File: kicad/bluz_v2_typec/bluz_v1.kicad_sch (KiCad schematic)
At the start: 76 parts, among them J10 Conn, J11 Conn, J12 BTAnt, J2 Conn, J3 Conn, J4 Conn, J5 Conn, J6 Conn, J7 Conn, J8 Conn, J9 USB_C_Receptacle_PowerOnly_6P, M1 Z3OC1T8219731, Q2 RUM002N05, SW1 SW_DPDT_x2, U1 MCP73831, U3 TLV3201AIDCK, U4 AP3015KTR, U5 MCP1700-1.8, U6 PAM8904EGPR, U7 TPS627451DSSR, Y1 NX1612SA-32MHz, Y2 NX2012SA-32.768

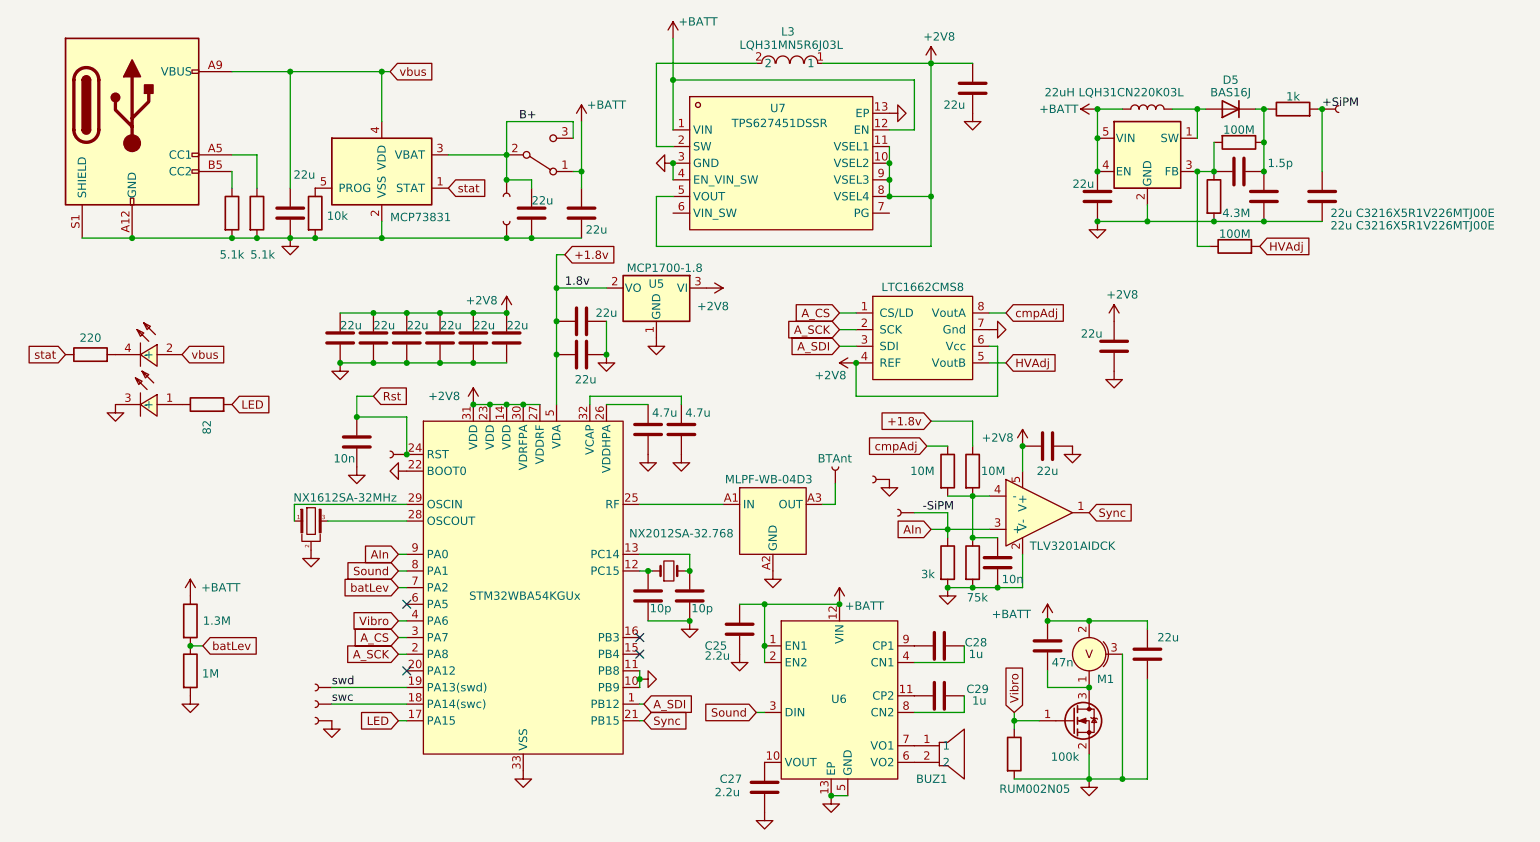
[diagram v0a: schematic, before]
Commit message: изменено:      Android/BluZ_v2/BluZ/Android/BluZ_LPM/BluZ/src/main/java/ru/starline/bluz/SettingsFragment.kt 	новый файл:    kicad/bluz_v1_LED/2024-05-07_07-39-39.kicad_sym 	новый файл:    kicad/bluz_v1_LED/CSPG6_1P05X1P65_STM-L.kicad_mod 	новый файл:    kicad/bluz_v1_LED/CSPG6_1P05X1P65_STM-M.kicad_mod 	новый файл:    kicad/bluz_v1_LED/CSPG6_1P05X1P65_STM.kicad_mod 	новый файл:    kicad/bluz_v1_LED/bluz_v1-backups/bluz_v1-2026-07-10_154057.zip 	новый файл:    kicad/bluz_v1_LED/bluz_v1-backups/bluz_v1-2026-07-10_154720.zip 	новый файл:    kicad/bluz_v1_LED/bluz_v1-backups/bluz_v1-2026-07-13_101334.zip 	новый файл:    kicad/bluz_v1_LED/bluz_v1-backups/bluz_v1-2026-07-13_113755.zip 	новый файл:    kicad/bluz_v1_LED/bluz_v1-backups/bluz_v1-2026-09-14_165340.zip 	новый файл:    kicad/bluz_v1_LED/bluz_v1-backups/bluz_v1-2026-09-14_165908.zip 	новый файл:    kicad/bluz_v1_LED/bluz_v1-backups/bluz_v1-2026-09-14_170418.zip 	новый файл:    kicad/bluz_v1_LED/bluz_v1-backups/bluz_v1-2026-09-14_174516.zip 	новый файл:    kicad/bluz_v1_LED/bluz_v1-backups/bluz_v1-2026-09-14_181225.zip 	новый файл:    kicad/bluz_v1_LED/bluz_v1-backups/bluz_v1-2026-09-15_141616.zip 	новый файл:    kicad/bluz_v1_LED/bluz_v1-backups/bluz_v1-2026-09-15_144107.zip 	новый файл:    kicad/bluz_v1_LED/bluz_v1-backups/bluz_v1-2026-09-15_145150.zip 	новый файл:    kicad/bluz_v1_LED/bluz_v1-backups/bluz_v1-2026-09-15_150420.zip 	новый файл:    kicad/bluz_v1_LED/bluz_v1-backups/bluz_v1-2026-09-15_155235.zip 	новый файл:    kicad/bluz_v1_LED/bluz_v1-backups/bluz_v1-2026-09-17_183048.zip 	новый файл:    kicad/bluz_v1_LED/bluz_v1-backups/bluz_v1-2026-09-17_183700.zip 	новый файл:    kicad/bluz_v1_LED/bluz_v1-backups/bluz_v1-2026-09-17_184420.zip 	новый файл:    kicad/bluz_v1_LED/bluz_v1-backups/bluz_v1-2026-09-17_185211.zip 	новый файл:    kicad/bluz_v1_LED/bluz_v1-backups/bluz_v1-2026-09-17_190709.zip 	новый файл:    kicad/bluz_v1_LED/bluz_v1-backups/bluz_v1-2026-09-18_172926.zip 	новый файл:    kicad/bluz_v1_L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
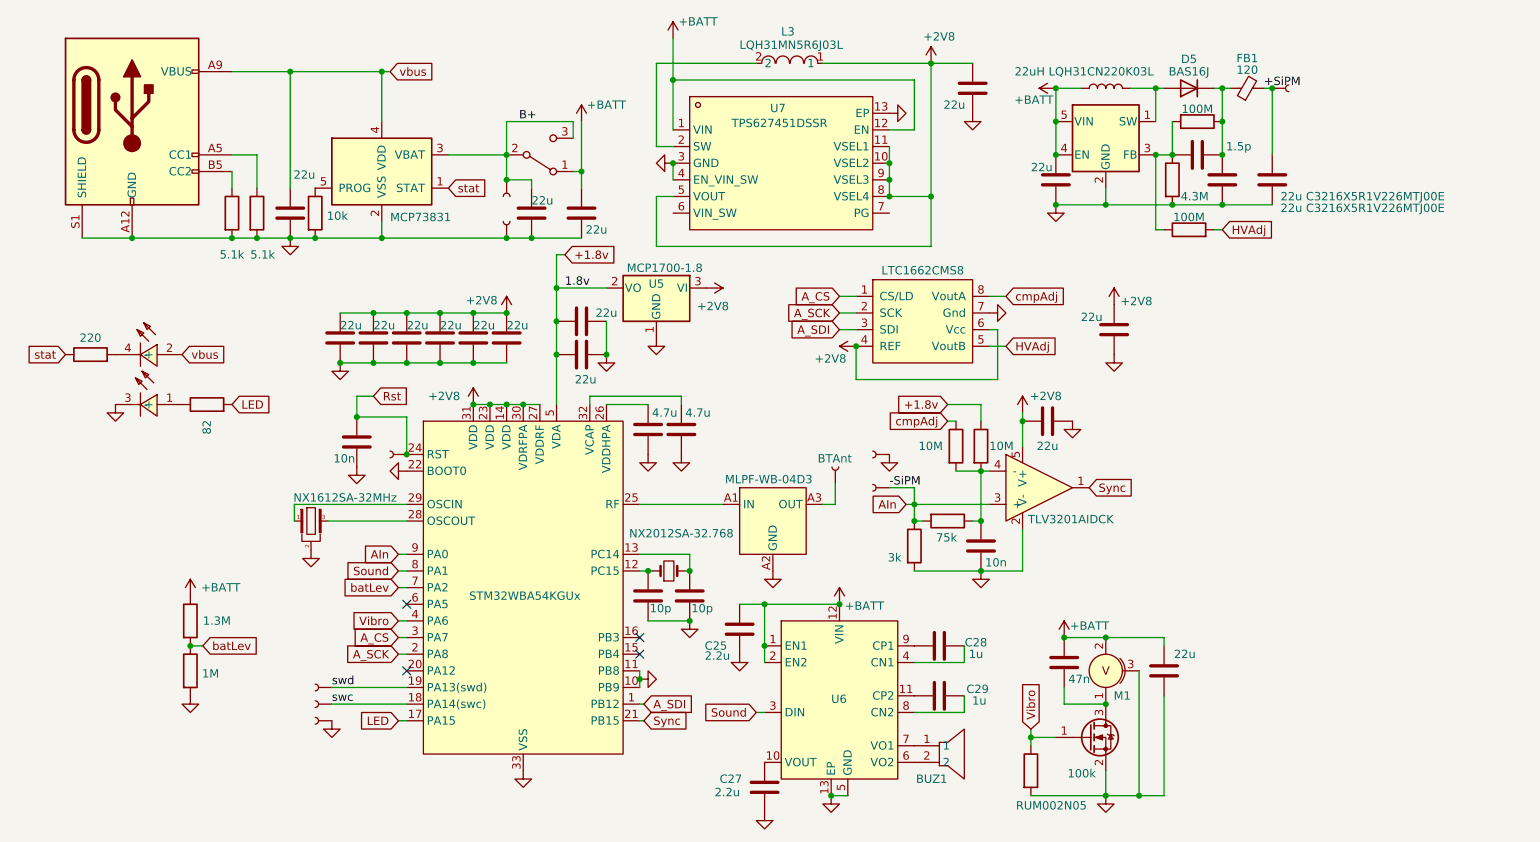
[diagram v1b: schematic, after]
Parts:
- removed R14: 1k, Resistor_SMD:R_0402_1005Metric, symbol Device:R
- added FB1: 120, Resistor_SMD:R_0402_1005Metric, symbol Device:FerriteBead_Small
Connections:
- net +SiPM: now also FB1.2
- net AIn: now also R10.2
- net GND: no longer R10.2
- net at C16.2, C9.1, D5.1 (K)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: now also FB1.1
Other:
- moved on the sheet: D5, M1
